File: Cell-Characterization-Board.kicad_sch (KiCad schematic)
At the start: 2 parts, among them IC2 INA4180A2IPWR, U1 ESP32-S3-WROOM-1

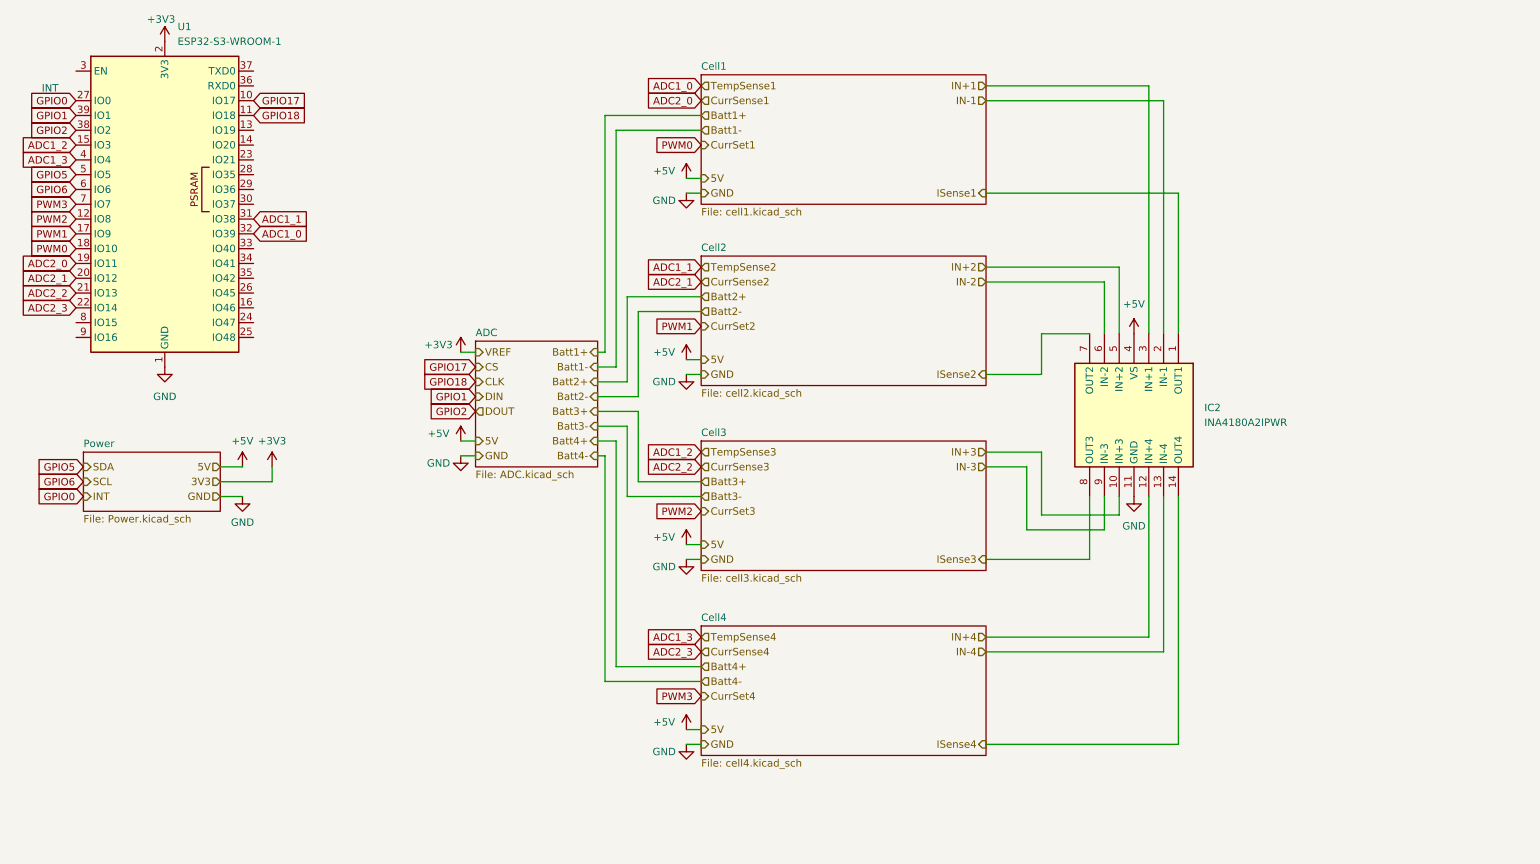
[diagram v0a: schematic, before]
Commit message: updated power stuff
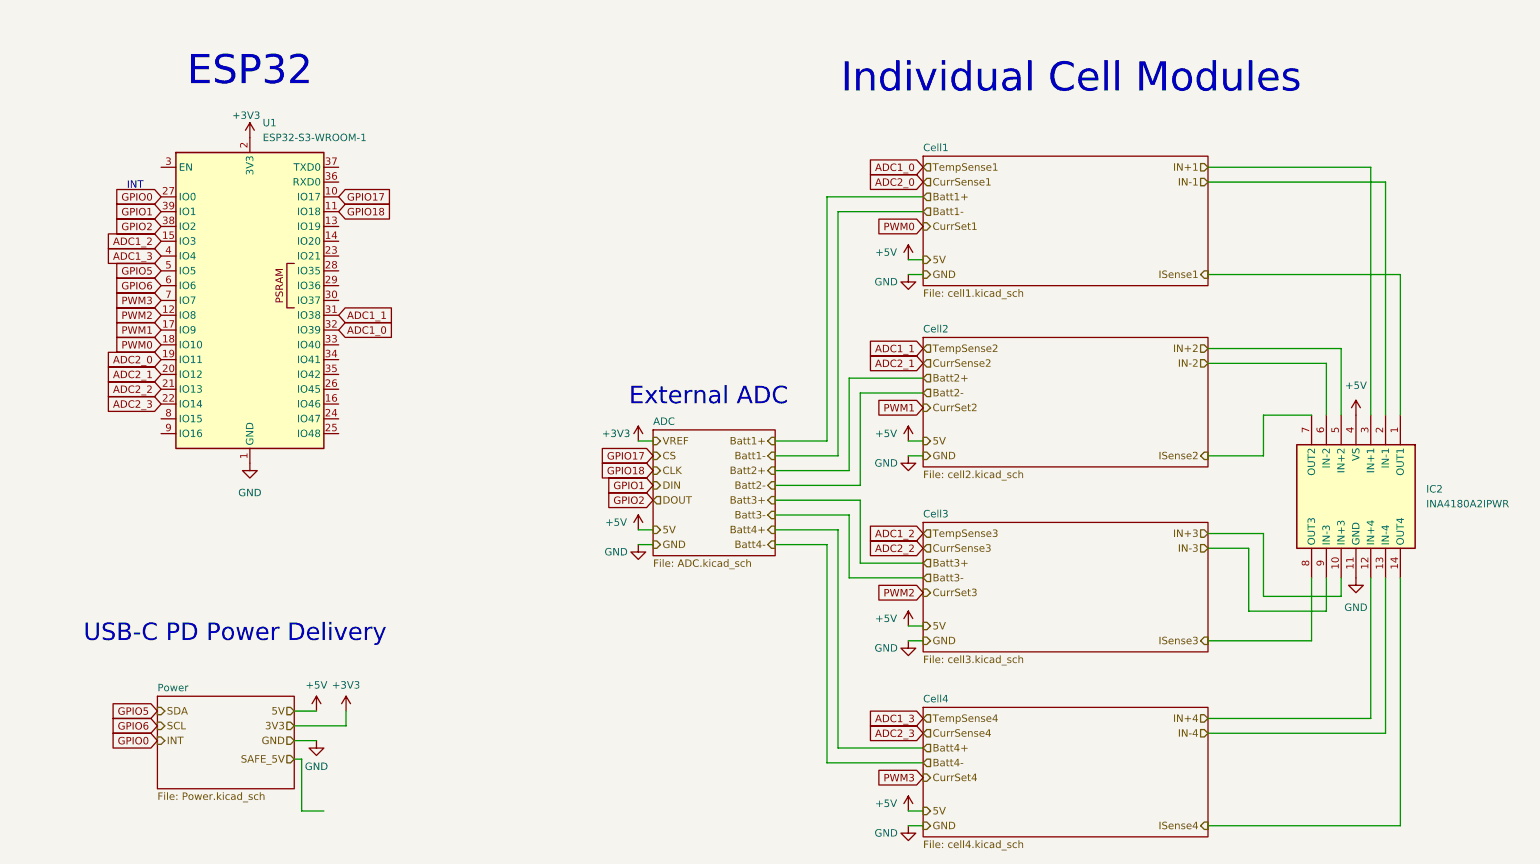
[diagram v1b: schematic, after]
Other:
- note added: "ESP32"
- note added: "External ADC"
- note added: "Individual Cell Modules"
- note added: "USB-C PD Power Delivery"
- moved on the sheet: IC2, U1
